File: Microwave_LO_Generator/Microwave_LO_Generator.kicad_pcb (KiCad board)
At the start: 4 copper layers, 52.5 x 42 mm, 76 parts, among them J1 Conn_01x02_Male, J2 Conn_01x02_Male, J3 Conn_01x02_Female, J4 Conn_01x05_Male, J5 Conn_01x02_Female, U1 ADF4150HV, U2 LT1962-3.3, U3 LT3010, U4 HMC739LP4E, U5 LT1962-5, U6 LT1962-5, X1 IQXT-220-1

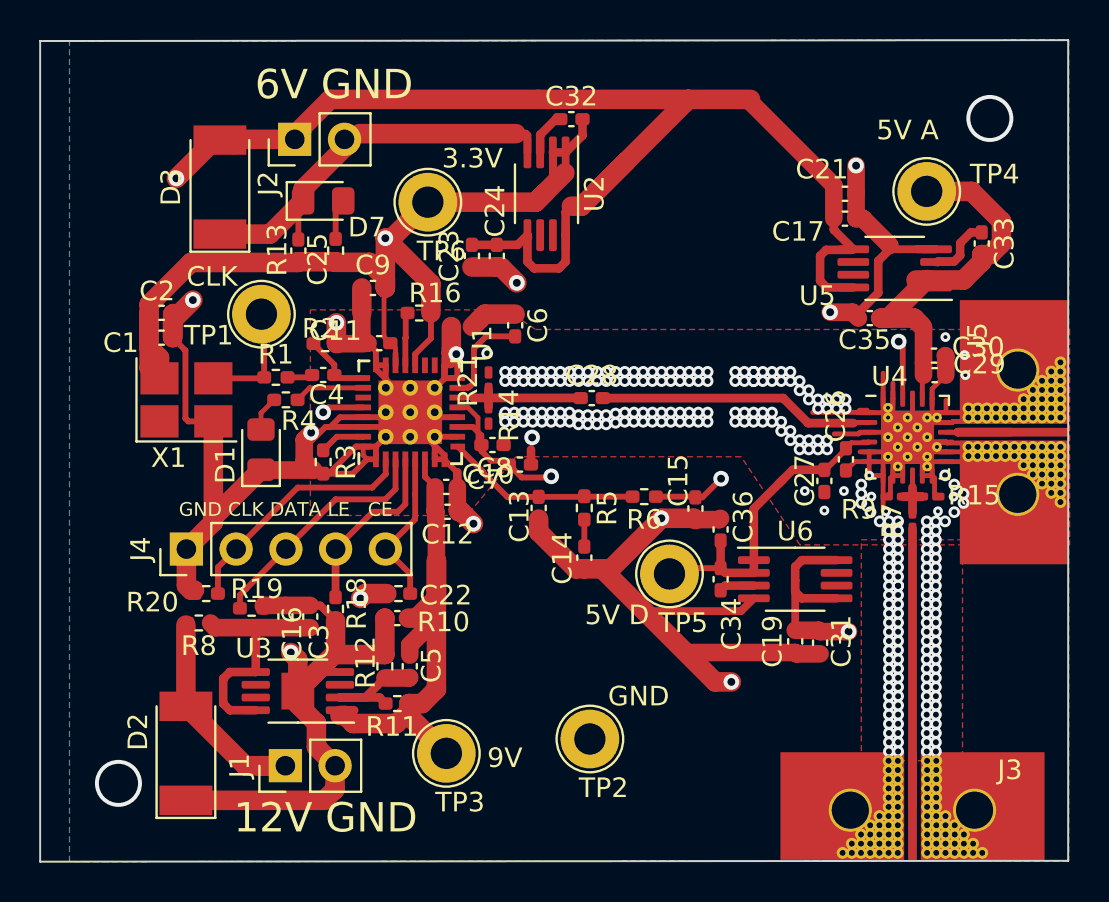
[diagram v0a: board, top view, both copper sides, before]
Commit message: some_update
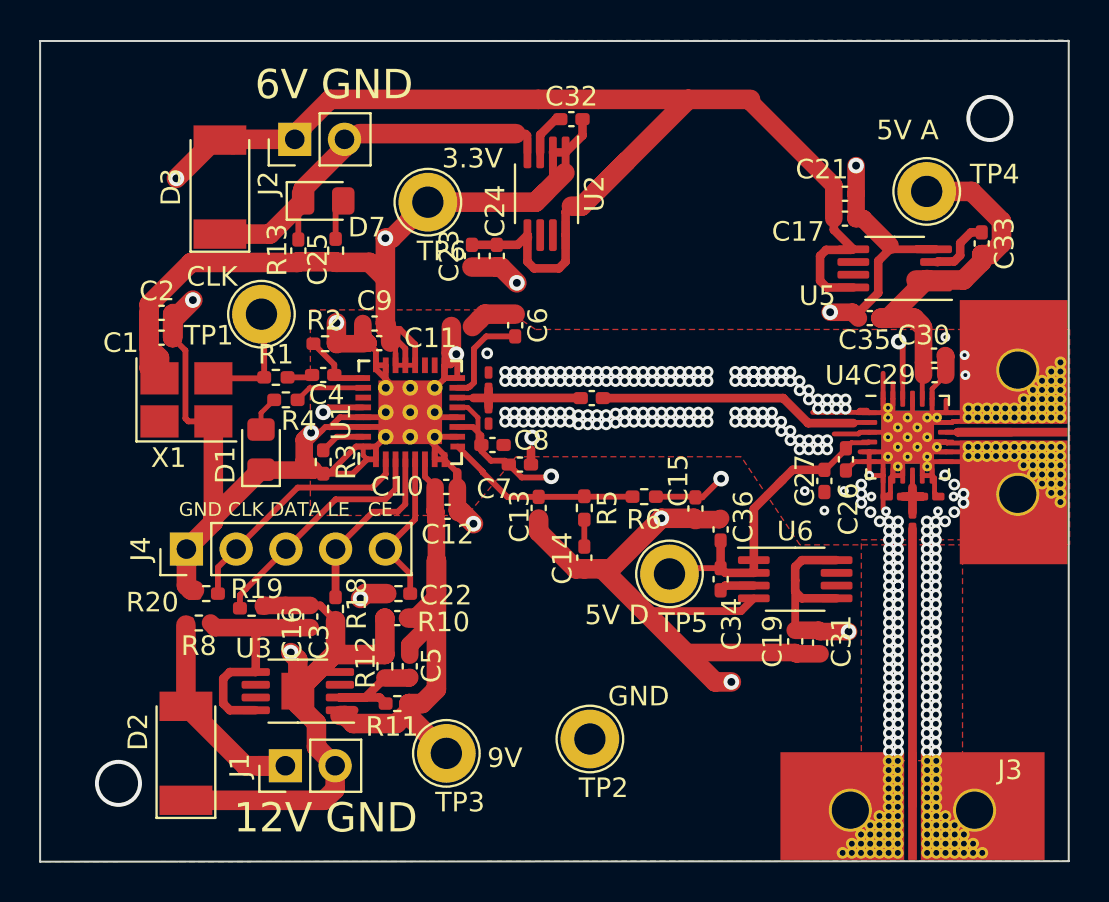
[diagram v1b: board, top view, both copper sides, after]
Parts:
- removed R16: 0, Resistor_SMD:R_0402_1005Metric_Pad0.72x0.64mm_HandSolder
- moved C9 1.82 mm to (106.5, 94.4)
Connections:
- U1 pad 21: Net-(R16-Pad2) -> +3V3
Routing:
- net +3V3: track 128.4 -> 123.9 mm
- net Net-(R16-Pad2): track 2.74 -> 0.00 mm
- net 0: track 276.5 -> 275.3 mm
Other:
- board size 52.5 x 42 mm -> 52.5 x 41.9 mm
